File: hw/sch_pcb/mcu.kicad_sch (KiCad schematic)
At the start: 40 parts, among them J2 SD_Card-FPS009-4200-0, J22 HEADER_2x03, J3 SM06B-GHS-TB, J4 SM04B-GHS-TB, SW2 MCU_RST, U10 ATMEGA1284P-AU, U11 PCF85263A, U6 AT24CS64-SSHM, Y1 8 MHz, Y2 ABS07-120-32.768KHZ-T

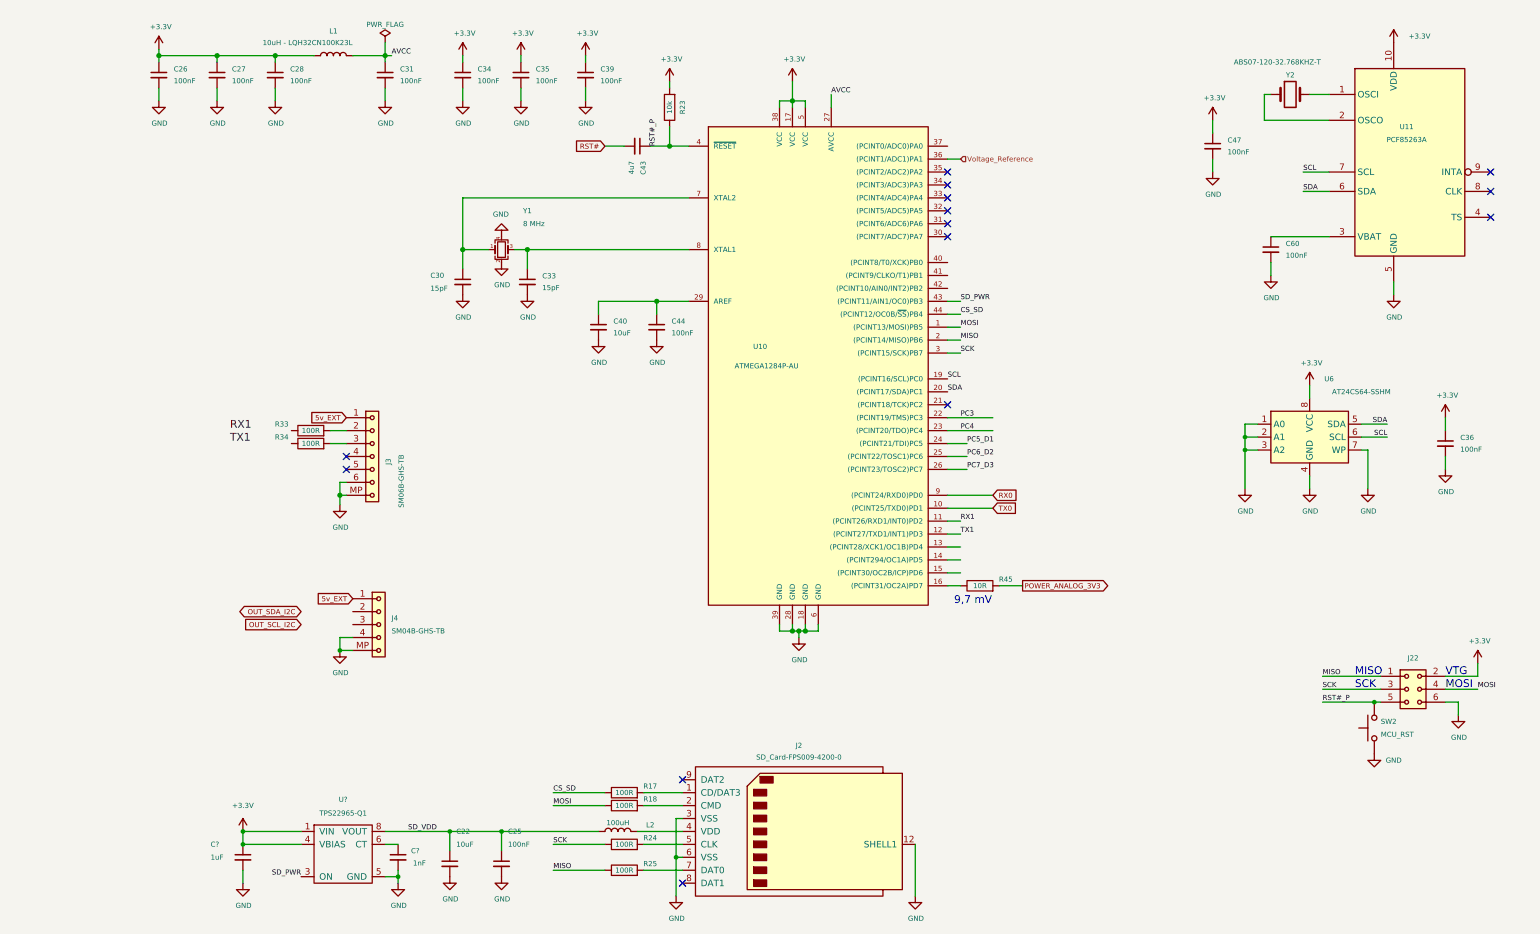
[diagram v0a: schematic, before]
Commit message: WIP: schematics and layout improvements
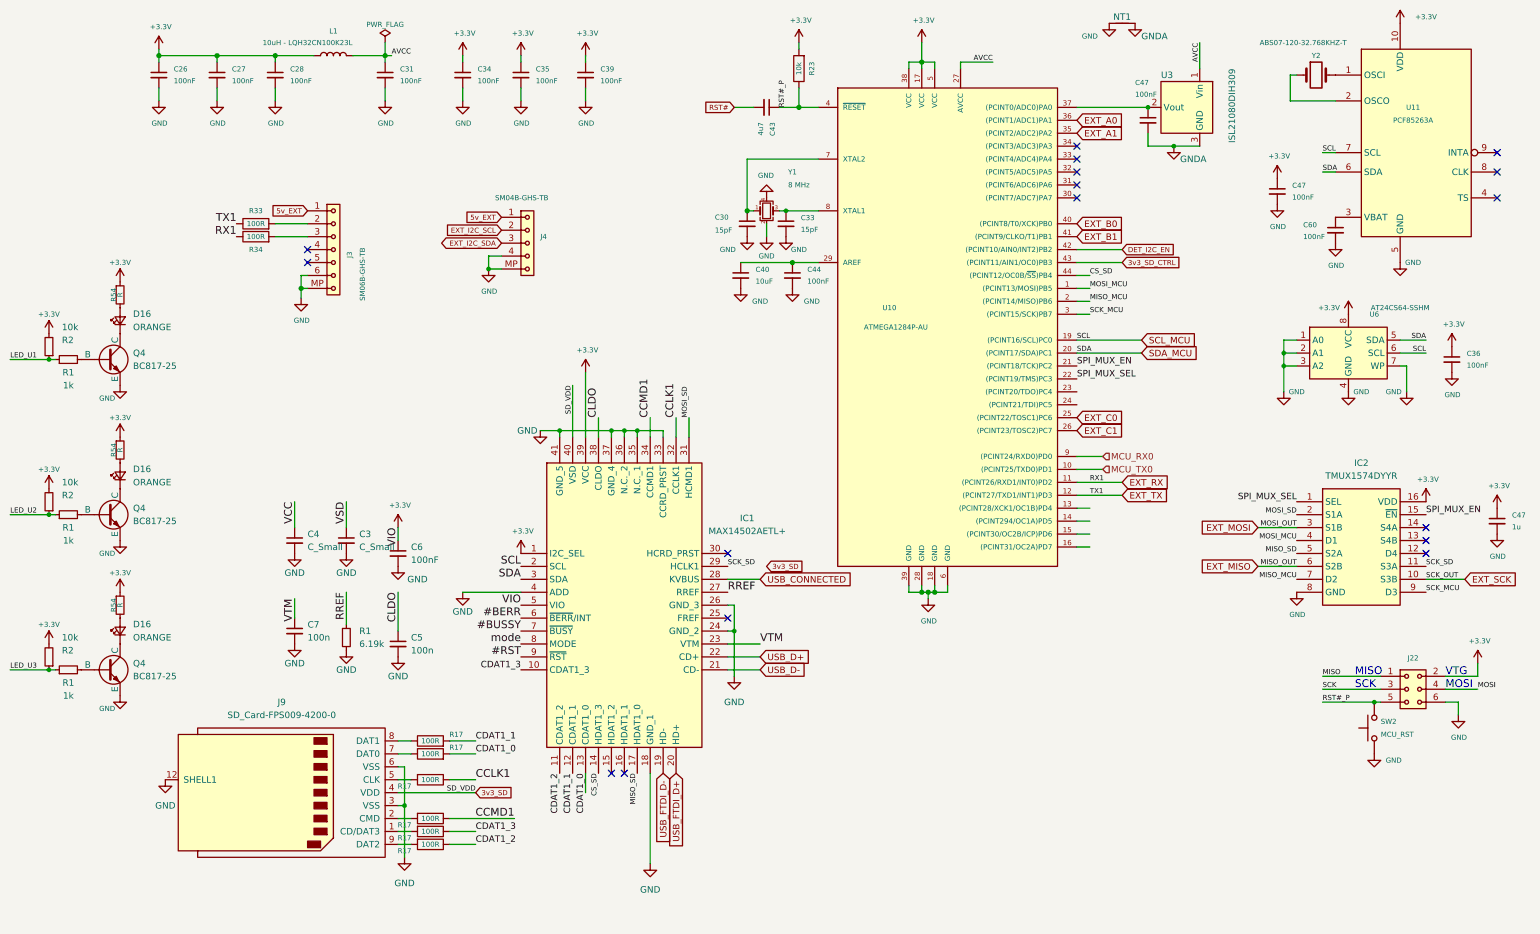
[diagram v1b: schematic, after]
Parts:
- removed C22: 10uF, Capacitor_SMD:C_0603_1608Metric, symbol Device:C_Small
- removed C25: 100nF, Capacitor_SMD:C_0805_2012Metric, symbol Device:C_Small
- removed C?: 1nF, Capacitor_SMD:C_0805_2012Metric, symbol Device:C_Small
- removed C?: 1uF, Capacitor_SMD:C_0805_2012Metric, symbol Device:C_Small
- removed J2: SD_Card-FPS009-4200-0, Mlab_CON:FPS009-4200-0, symbol MLAB_CONNECTORS:SD_Card-FPS009-4200-0
- removed L2: 100uH, Inductor_SMD:L_0805_2012Metric_Pad1.15x1.40mm_HandSolder, symbol Device:L
- removed R17, R18, R24, R25: 100R, Resistor_SMD:R_0805_2012Metric, symbol SPACEDOS02A_PCB01A-rescue:R-device-DATALOGGER01A-rescue-CCP2019V01A-rescue-SPAC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
- removed R45: 10R, Resistor_SMD:R_0805_2012Metric, symbol SPACEDOS02A_PCB01A-rescue:R-device-DATALOGGER01A-rescue-CCP2019V01A-rescue-SPAC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
- removed U?: TPS22965-Q1, Package_SON:WSON-8-1EP_2x2mm_P0.5mm_EP0.9x1.6mm_ThermalVias, symbol DATALOGGER01A-rescue:TPS22965-Q1-MLAB_IO
- added C3, C4: C_Small, Capacitor_SMD:C_0805_2012Metric, symbol Device:C_Small
- added C47, C6: 100nF, Capacitor_SMD:C_0805_2012Metric, symbol Device:C_Small
- added C47: 1u, Capacitor_SMD:C_0805_2012Metric, symbol Device:C_Small
- added C5, C7: 100n, Capacitor_SMD:C_0805_2012Metric, symbol Device:C_Small
- added D16 (x3): ORANGE, LED_SMD:LED_1206_3216Metric, symbol Device:LED_Small
- added IC1: MAX14502AETL+, Mlab_IO:QFN40P500X500X80-41N, symbol MLAB_IO:MAX14502AETL+
- added IC2: TMUX1574DYYR, symbol MLAB_IO:TMUX1574DYYR
- added J9: SD_Card-FPS009-4200-0, Mlab_CON:FPS009-4200-0, symbol MLAB_CONNECTORS:SD_Card-FPS009-4200-0
- added NT1: NetTie_2, NetTie:NetTie-2_SMD_Pad0.5mm, symbol Device:NetTie_2
- added Q4 (x3): BC817-25, Package_TO_SOT_SMD:SOT-23-3, symbol Simulation_SPICE:NPN
- added R1 (x3): 1k, Resistor_SMD:R_0805_2012Metric, symbol Device:R_Small
- added R1: 6.19k, Resistor_SMD:R_0805_2012Metric, symbol Device:R_Small
- added R17 (x6): 100R, Resistor_SMD:R_0805_2012Metric, symbol SPACEDOS02A_PCB01A-rescue:R-device-DATALOGGER01A-rescue-CCP2019V01A-rescue-SPAC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
- added R2 (x3): 10k, Resistor_SMD:R_0805_2012Metric, symbol Device:R_Small
- added R54 (x3): R, Resistor_SMD:R_0805_2012Metric, symbol Device:R_Small
- added U3: ISL21080DIH309, Package_TO_SOT_SMD:SOT-23, symbol Reference_Voltage:ISL21070CIH320Z-TK
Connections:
- net RX1 is gone; now on net EXT_RX: U10.11 ((PCINT26/RXD1/INT0)PD2)
- net TX1 is gone; now on net EXT_TX: U10.12 ((PCINT27/TXD1/INT1)PD3)
- net +3.3V: now also C47.1, C6.1, IC1.1 (I2C_SEL), IC1.39 (VCC), IC1.5 (VIO), IC2.16 (VDD), R2.2, R2.2, R2.2, R54.1, R54.1, R54.1
- net AVCC: now also U3.1 (Vin)
- net CS_SD: now also IC1.14 (HDAT1_3)
- net GND: now also C3.2, C4.2, C47.2, C5.2, C6.2, C7.2, IC1.18 (GND_1), IC1.24 (GND_2), IC1.26 (GND_3), IC1.33 (CCRD_PRST), IC1.35 (N.C._1), IC1.36 (N.C._2), IC1.37 (GND_4), IC1.4 (ADD), IC1.41 (GND_5), IC2.8 (GND), J9.12 (SHELL1), J9.3 (VSS), J9.6 (VSS), NT1.1, Q4.3 (E), Q4.3 (E), Q4.3 (E), R1.2
- net MISO: no longer U10.2 ((PCINT14/MISO)PB6)
- net MOSI: no longer U10.1 ((PCINT13/MOSI)PB5)
- net SCK: no longer U10.3 ((PCINT15/SCK)PB7)
- net EXT_I2C_SCL: now reaches J4.2
- net EXT_I2C_SDA: now reaches J4.3
- net EXT_RX: now reaches R34.1
- net SPI_MUX_EN: now reaches U10.21 ((PCINT18/TCK)PC2)
- net SPI_MUX_EN: now also IC2.15 (~{EN})
- net EXT_A1: now reaches U10.35 ((PCINT2/ADC2)PA2)
- net at U10.37 ((PCINT0/ADC0)PA0): now also C47.1, U3.2 (Vout)
- net EXT_B0: now reaches U10.40 ((PCINT8/T0/XCK)PB0)
- net EXT_B1: now reaches U10.41 ((PCINT9/CLKO/T1)PB1)
- net DET_I2C_EN: now reaches U10.42 ((PCINT10/AIN0/INT2)PB2)
- net EXT_TX: now reaches R33.1
- net PC3 renamed SPI_MUX_SEL
- net SPI_MUX_SEL: now also IC2.1 (SEL)
- net PC4: no longer names the net of U10.23 ((PCINT20/TDO)PC4)
- net PC5_D1: no longer names the net of U10.24 ((PCINT21/TDI)PC5)
- net PC6_D2 renamed EXT_C0
- net PC7_D3 renamed EXT_C1
- net RX0 renamed MCU_RX0
- net SCL renamed SCL_MCU
- net SCL_MCU: now also IC1.2 (SCL)
- net SDA renamed SDA_MCU
- net SDA_MCU: now also IC1.3 (SDA)
- net SD_PWR renamed 3v3_SD_CTRL
- net TX0 renamed MCU_TX0
- net Voltage_Reference renamed EXT_A0
- new net: D16.2 (A), R54.2 (x3)
- new net: J9.9 (DAT2), R17.2
- new net: J9.1 (CD/DAT3), R17.2
- new net: J9.2 (CMD), R17.2
- new net: J9.5 (CLK), R17.2
- new net: J9.7 (DAT0), R17.1
- new net: J9.8 (DAT1), R17.1
- new net: D16.1 (K), Q4.1 (C) (x3)
- new net: Q4.2 (B), R1.2 (x3)
- new net #BERR: IC1.6 (~{BERR}/INT)
- new net #BUSSY: IC1.7 (~{BUSY})
- new net #RST: IC1.9 (~{RST})
- new net 3v3_SD: IC1.40 (VSD), J9.4 (VDD)
- new net CCLK1: IC1.32 (CCLK1), R17.1
- new net CCMD1: IC1.34 (CCMD1), R17.1
- new net CDAT1_0: IC1.13 (CDAT1_0), R17.2
- new net CDAT1_1: IC1.12 (CDAT1_1), R17.2
- new net CDAT1_2: IC1.11 (CDAT1_2), R17.1
- new net CDAT1_3: IC1.10 (CDAT1_3), R17.1
- new net CLDO: C5.1, IC1.38 (CLDO)
- new net EXT_MISO: IC2.6 (S2B)
- new net EXT_MOSI: IC2.3 (S1B)
- new net EXT_SCK: IC2.10 (S3B)
- new net GNDA: C47.2, NT1.2, U3.3 (GND)
- new net LED_U1: R1.1, R2.1
- new net LED_U2: R1.1, R2.1
- new net LED_U3: R1.1, R2.1
- new net MISO_MCU: IC2.7 (D2), U10.2 ((PCINT14/MISO)PB6)
- new net MISO_SD: IC1.17 (HDAT1_0), IC2.5 (S2A)
- new net MOSI_MCU: IC2.4 (D1), U10.1 ((PCINT13/MOSI)PB5)
- new net MOSI_SD: IC1.31 (HCMD1), IC2.2 (S1A)
- new net RREF: IC1.27 (RREF), R1.1
- new net SCK_MCU: IC2.9 (D3), U10.3 ((PCINT15/SCK)PB7)
- new net SCK_SD: IC1.29 (HCLK1), IC2.11 (S3A)
- new net USB_CONNECTED: IC1.28 (KVBUS)
- new net USB_D+: IC1.22 (CD+)
- new net USB_D-: IC1.21 (CD-)
- new net USB_FTDI_D+: IC1.20 (HD+)
- new net USB_FTDI_D-: IC1.19 (HD-)
- new net VCC: C4.1
- new net VSD: C3.1
- new net VTM: C7.1, IC1.23 (VTM)
- new net mode: IC1.8 (MODE)
- no-connect marks 14 -> 17
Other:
- note removed: "9,7 mV"
- moved on the sheet: C30, C33, C36, C40, C43, C44, C47, C60, J3, J4, R23, R33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
